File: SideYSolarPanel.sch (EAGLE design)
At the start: 33 parts

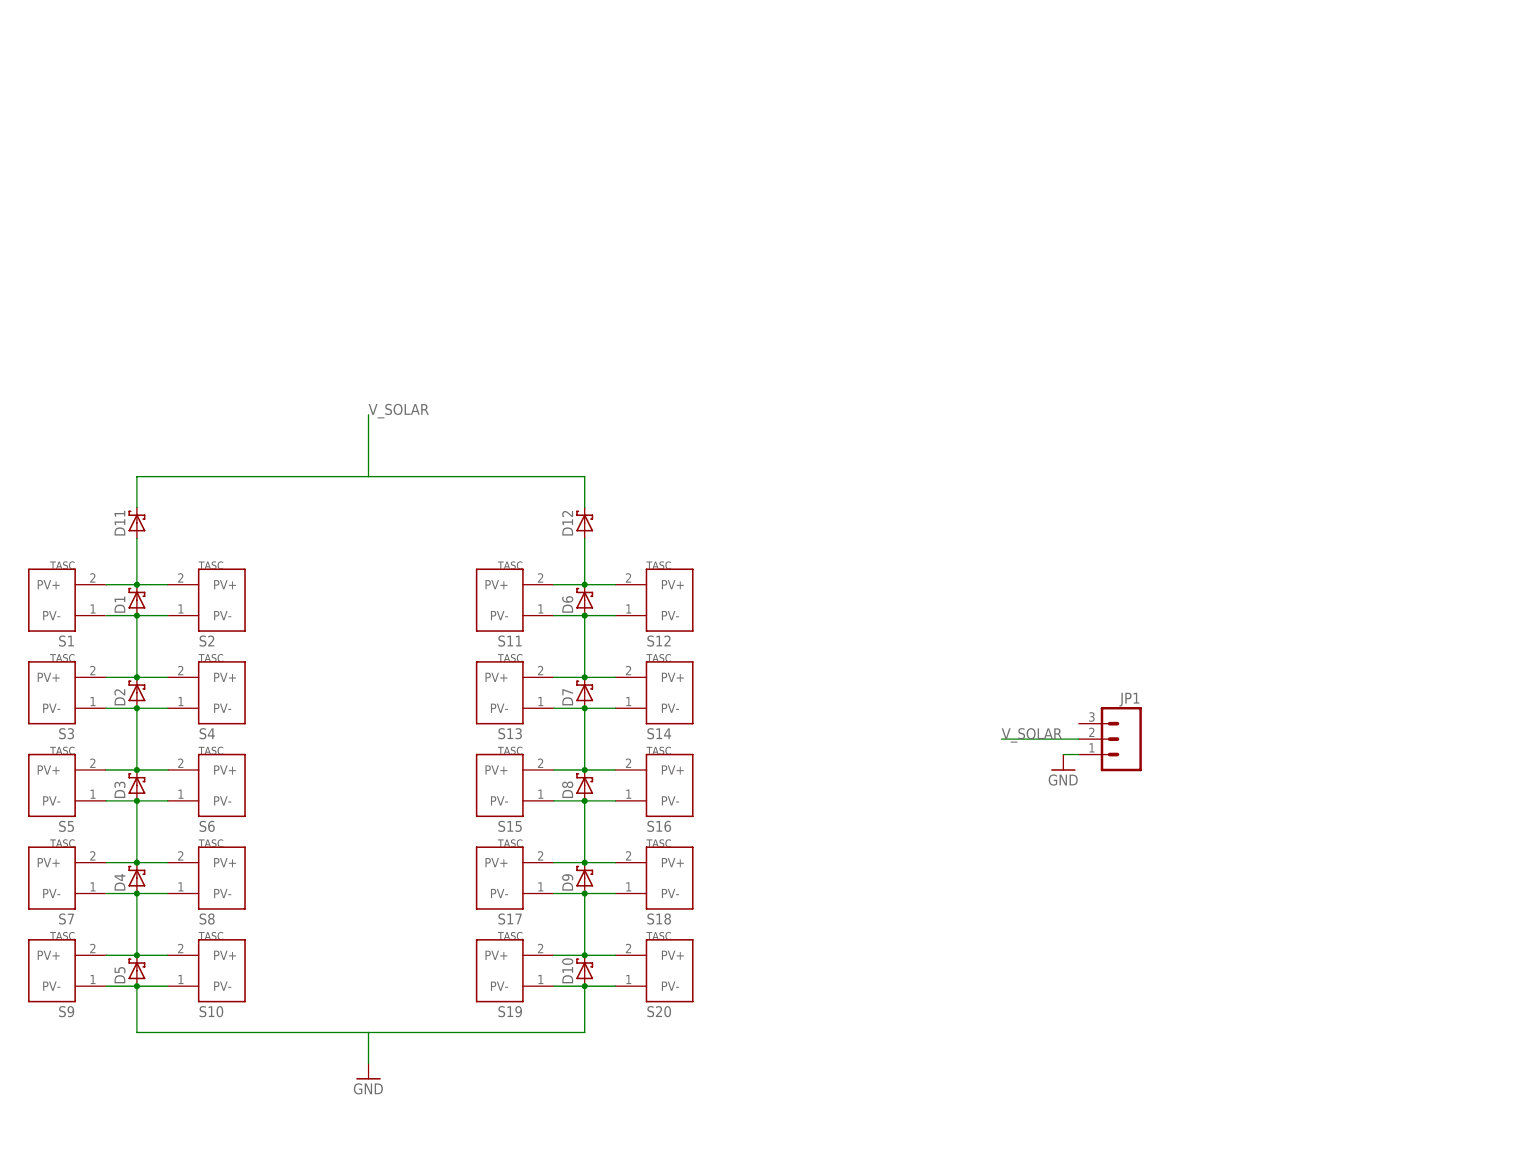
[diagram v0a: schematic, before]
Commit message: Cleanup
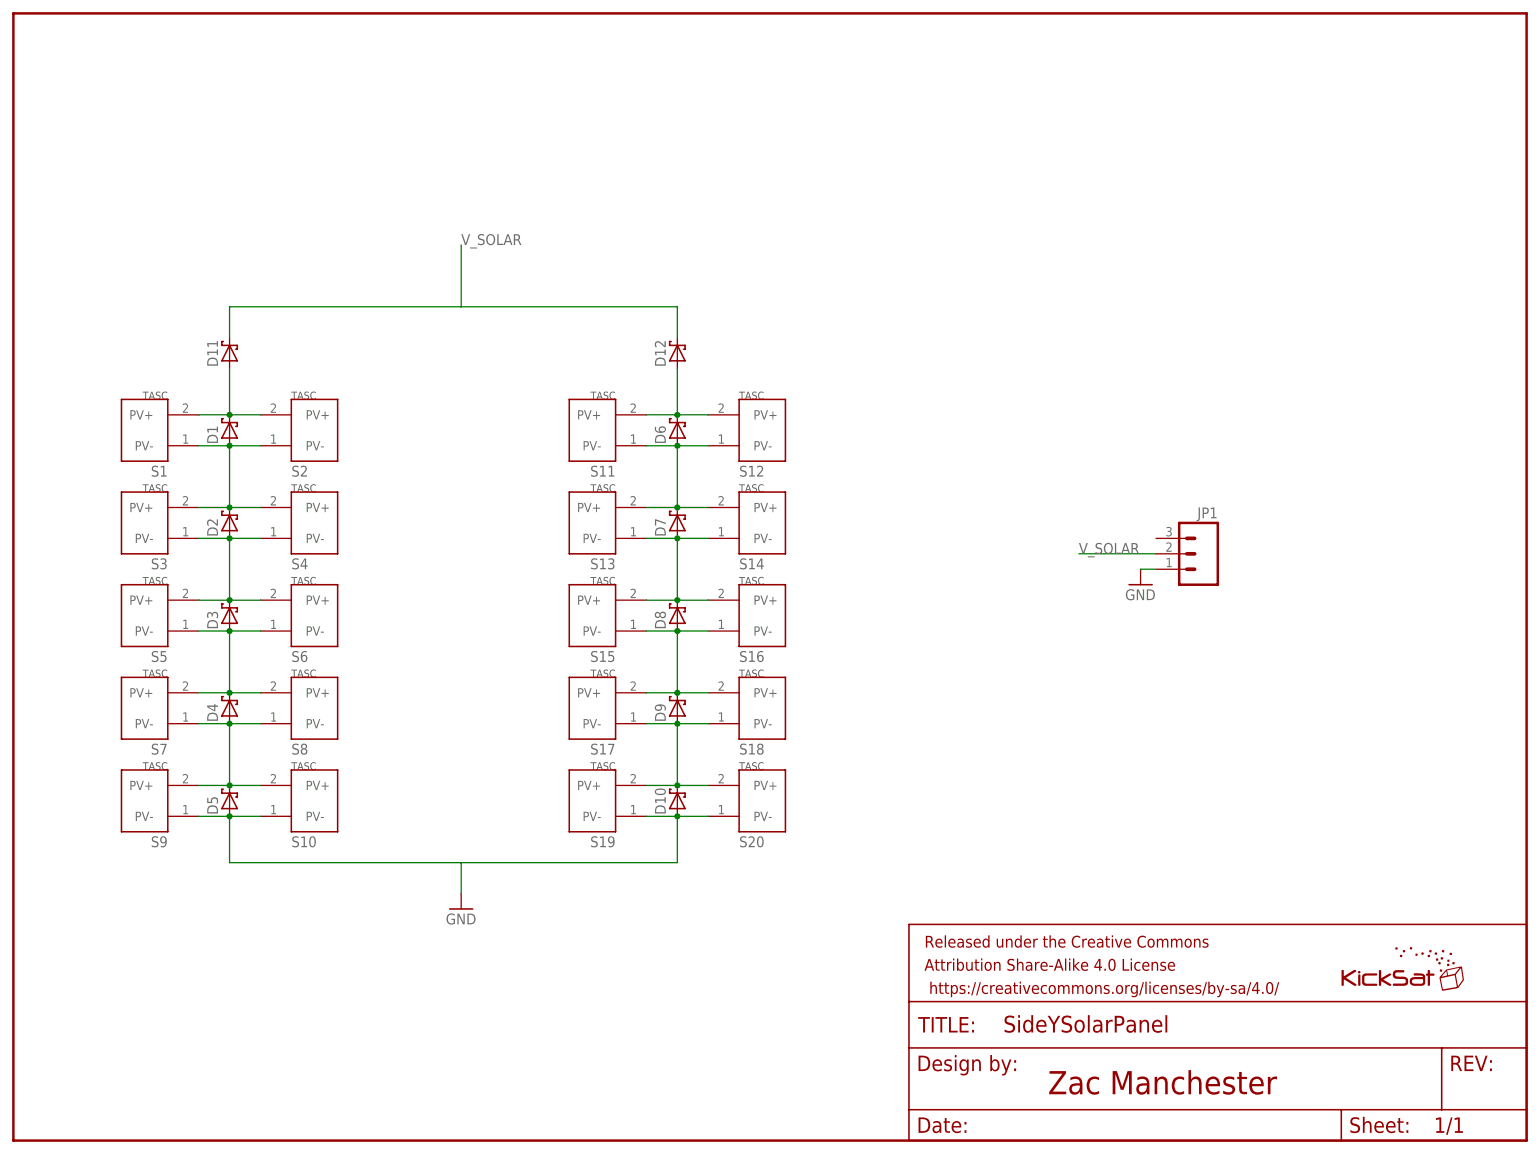
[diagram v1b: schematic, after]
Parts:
- added FRAME1: FRAME-LETTER, SparkFun-Aesthetics:FRAME-LETTER
- added U$1: KICKSAT_LOGO, KickSat-Logo:KICKSAT_LOGO
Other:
- note added: "Zac Manchester"
- moved on the sheet: D1, D10, D11, D12, D2, D3, D4, D5, D6, D7, D8, D9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
